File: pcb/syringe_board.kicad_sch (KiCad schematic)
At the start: 35 parts, among them J1 54602-908LF, J2 ESQ-116-12-T-S, J3 ESQ-112-12-T-S, J4 PH1RB-07-UA, J5 Conn_02x03_Odd_Even, J6 Motor leads, J7 PPTC071LGBN-RC, J8 Limit switches, U1 BU33SD2MG, U2 ATSAMD21G, U3 TMC2209, U4 AT24C01C-STUM, X1 feather_wing

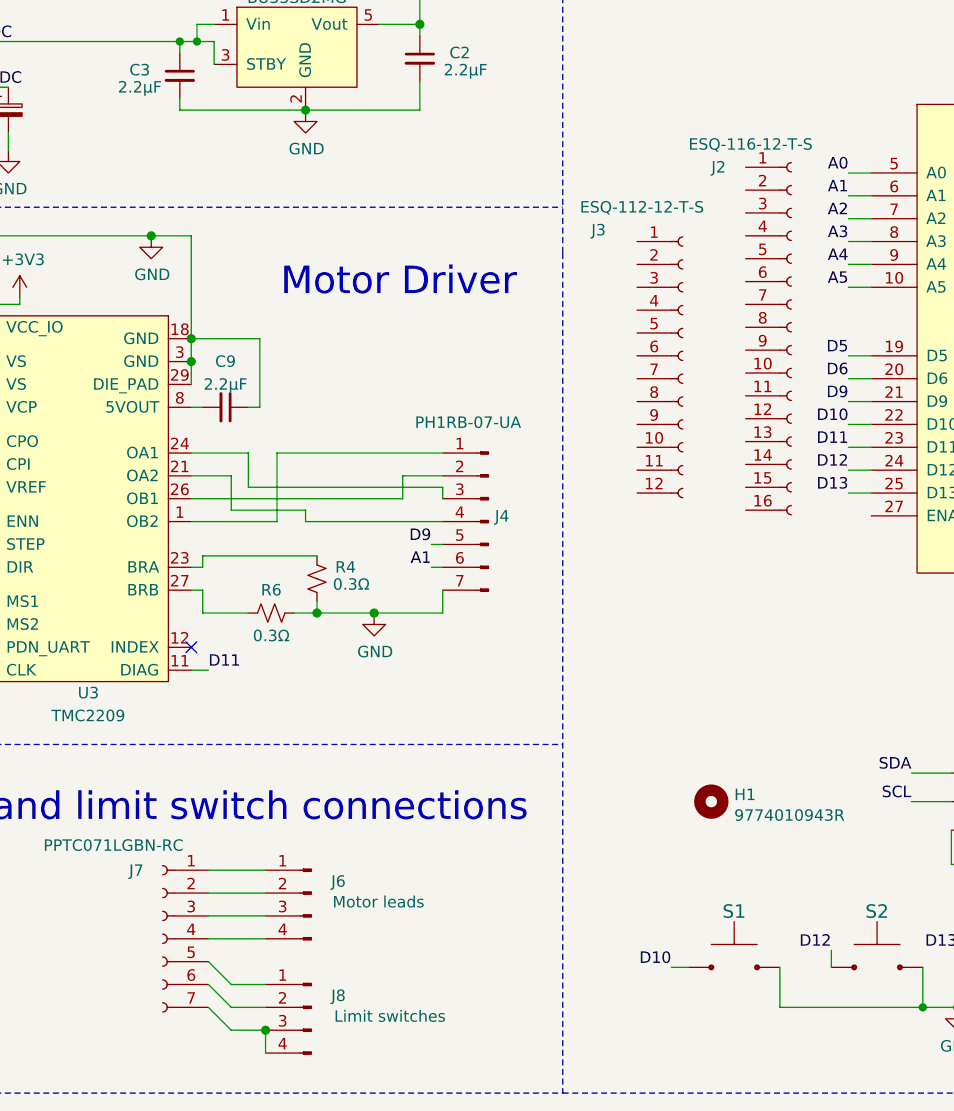
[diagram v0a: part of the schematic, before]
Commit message: up to date CAD
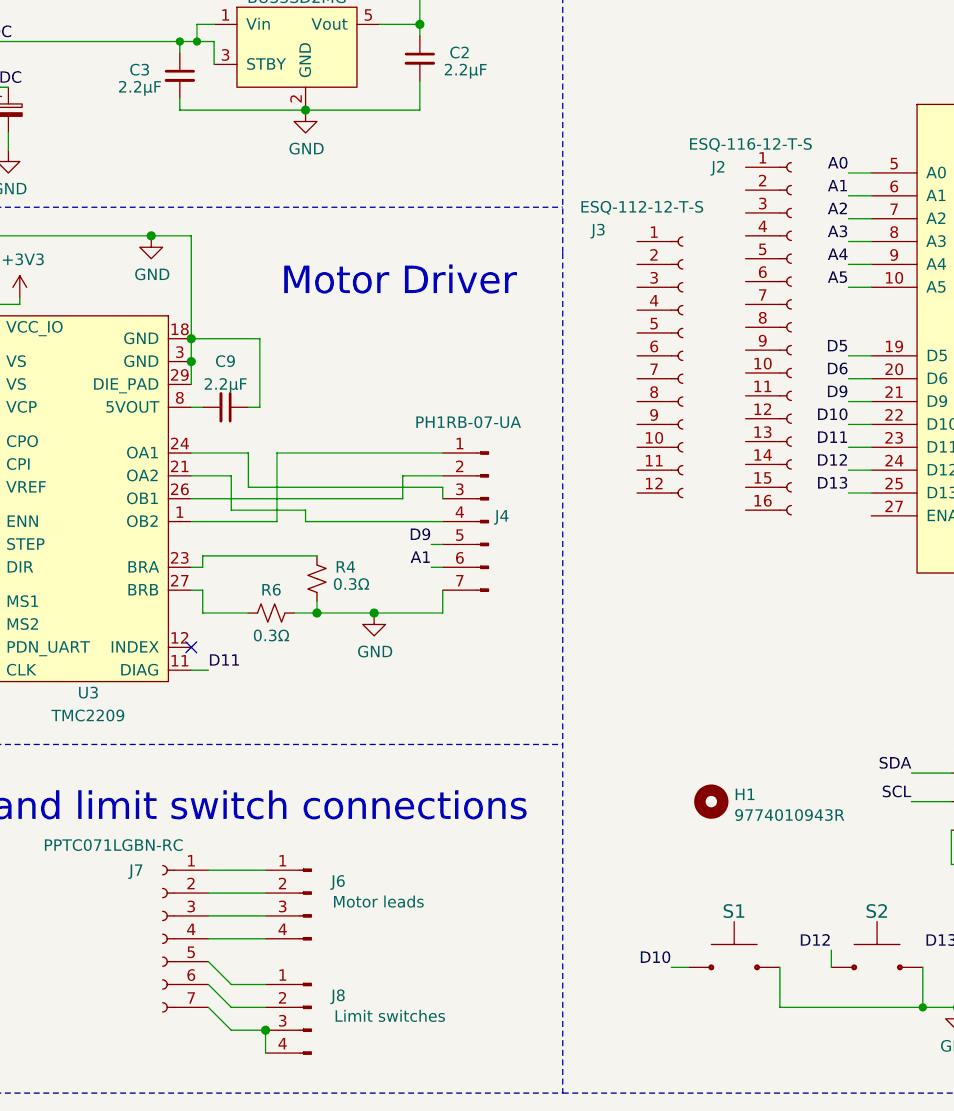
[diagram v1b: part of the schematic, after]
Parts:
- J1: footprint asl_footprints:RJ45_THP_Vertical -> asl_footprints:RJ45_THP
